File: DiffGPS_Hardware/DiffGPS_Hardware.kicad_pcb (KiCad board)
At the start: 2 copper layers, 110.2 x 72.3 mm, 16 parts, among them U1 Raspberry_Pi

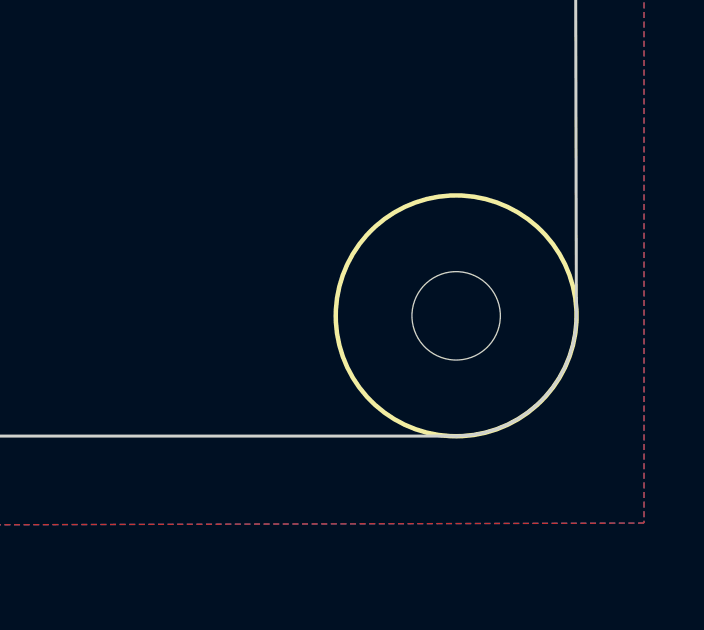
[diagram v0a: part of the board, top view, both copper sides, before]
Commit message: finished GERBS
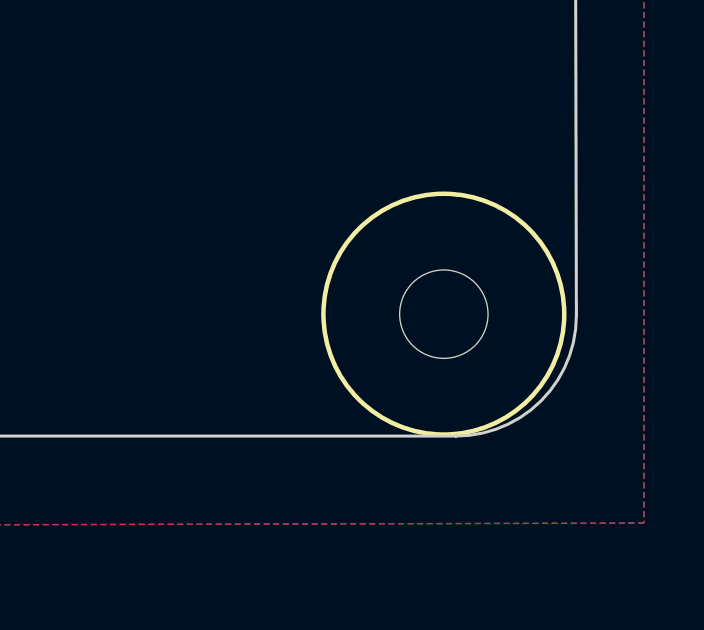
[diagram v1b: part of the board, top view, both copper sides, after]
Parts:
- moved H3 0.41 mm to (155.7, 114.2)
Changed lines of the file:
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@@
       (drillshape 0)
       (scaleselection 1)
-      (outputdirectory "../Manufacturing/")
+      (outputdirectory "../Manufacturing/Gerbs/")
     )
   )
@@
   )
   (footprint "MRDT_Drill_Holes:4_40_Hole_Corner" (layer "F.Cu")
-    (at 156.0757 114.3 90)
+    (at 155.6653 114.24412 90)
     (property "Sheetfile" "DiffGPS_Hardware.kicad_sch")
     (property "Sheetname" "")
